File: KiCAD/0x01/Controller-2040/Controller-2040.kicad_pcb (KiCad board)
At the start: 2 copper layers, 45 x 69 mm, 3 parts, among them J1 pots-conn, J2 enc-conn

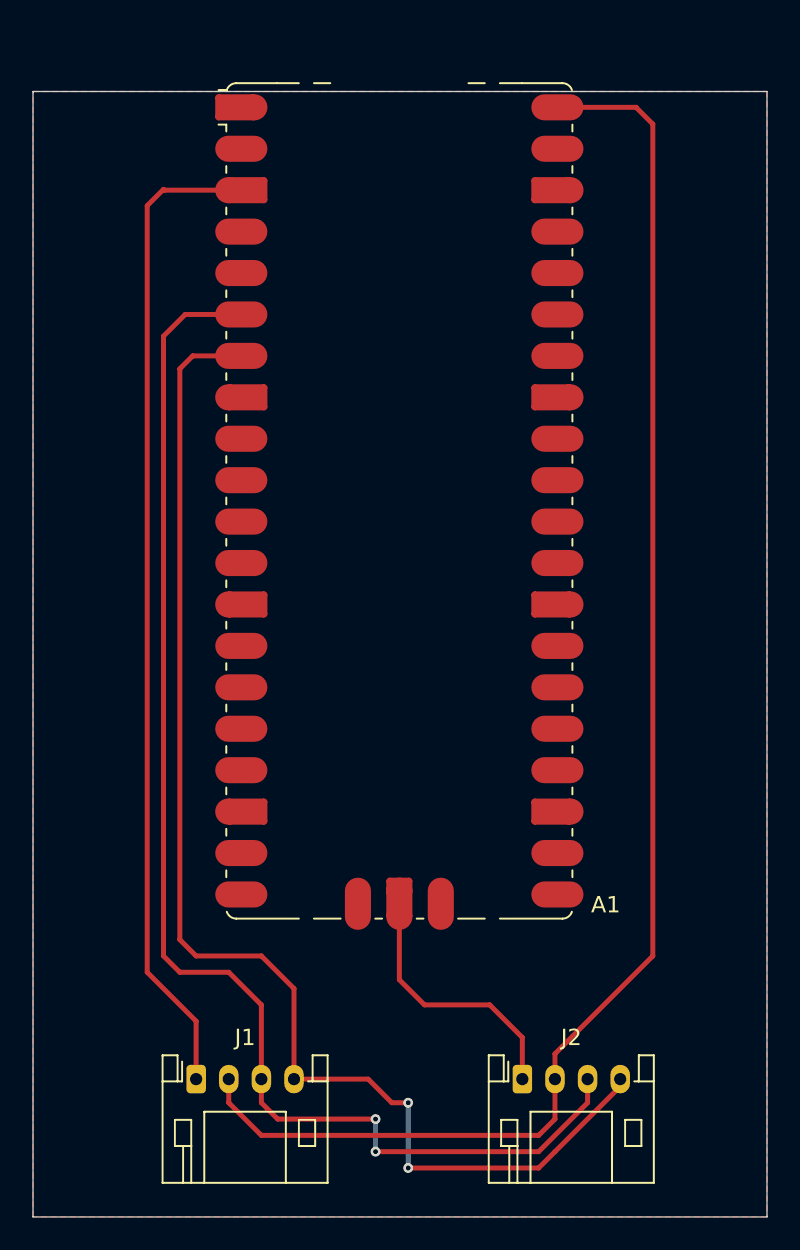
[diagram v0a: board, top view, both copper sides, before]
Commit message: rp2040 zero
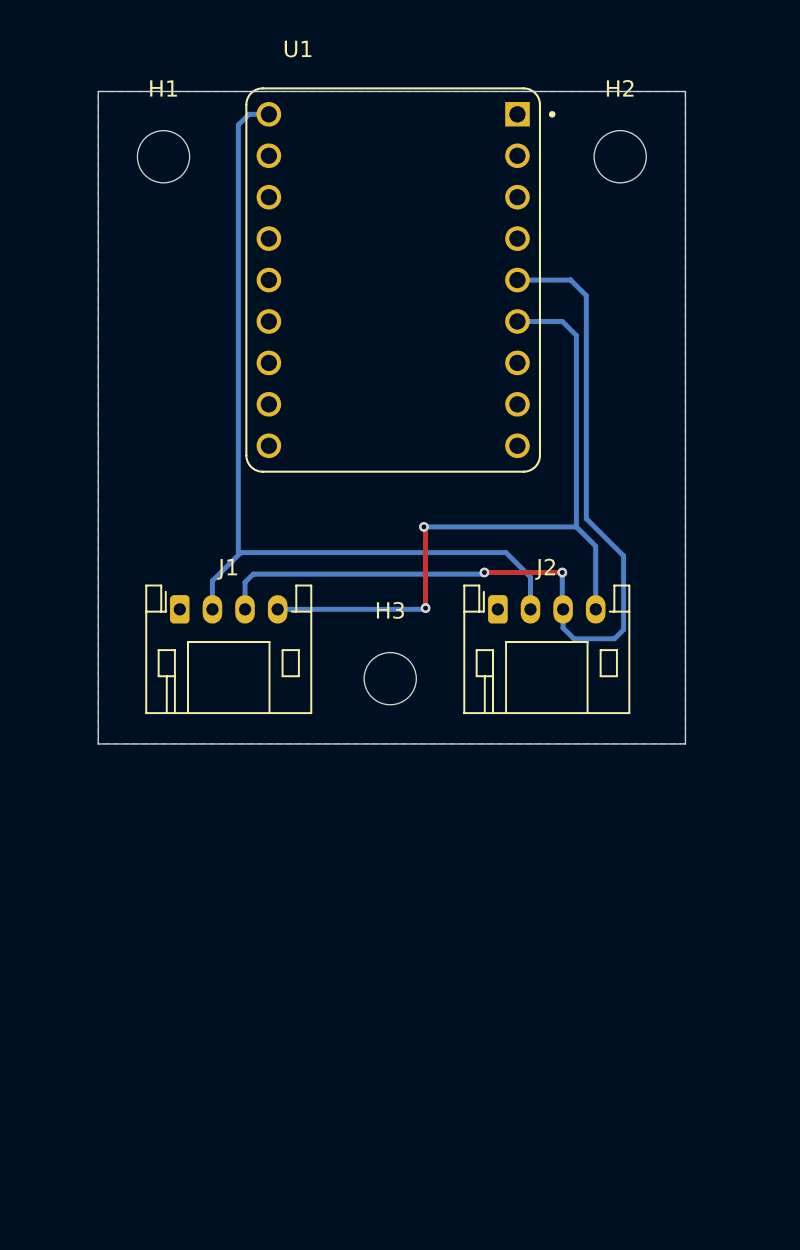
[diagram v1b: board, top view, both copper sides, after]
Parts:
- removed A1: RaspberryPi_Pico, Module:RaspberryPi_Pico_SMD
- added H1: MountingHole, MountingHole:MountingHole_3.2mm_M3, F.Cu at (93.0, 50.0)
- added H2: MountingHole, MountingHole:MountingHole_3.2mm_M3, F.Cu at (121.0, 50.0)
- added H3: MountingHole, MountingHole:MountingHole_3.2mm_M3, F.Cu at (106.9, 82.0)
- added U1: RP2040-ZERO, 2040Library:MODULE_RP2040-ZEROa, F.Cu at (107.1, 57.6)
- moved J2 28.8 mm to (113.5, 77.8)
- moved J1 28.8 mm to (94.0, 77.8)
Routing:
- net /GND: track 78.0 -> 0.00 mm
- net /VCC: track 92.5 -> 53.0 mm
- net /SCL: track 80.0 -> 44.7 mm
- net /SDA: track 81.7 -> 55.0 mm
- added copper zone on B.Cu, net /GND
- removed copper zone on F.Cu, net /GND
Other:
- board size 45 x 69 mm -> 36 x 40 mm
